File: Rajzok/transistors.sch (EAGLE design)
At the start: 17 parts, among them Q1 TP0602N2, Q2 TP0602N2, Q3 SUP75N06-08, Q4 SUP75N06-08

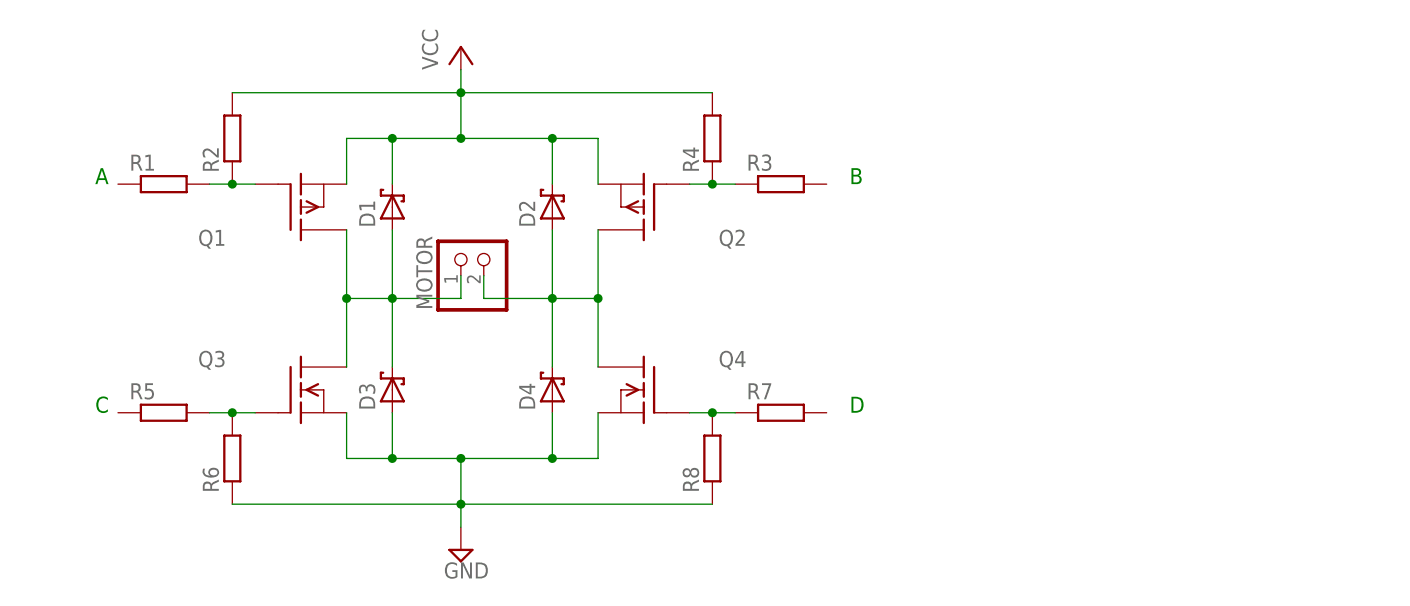
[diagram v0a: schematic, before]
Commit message: Rajzok 2017
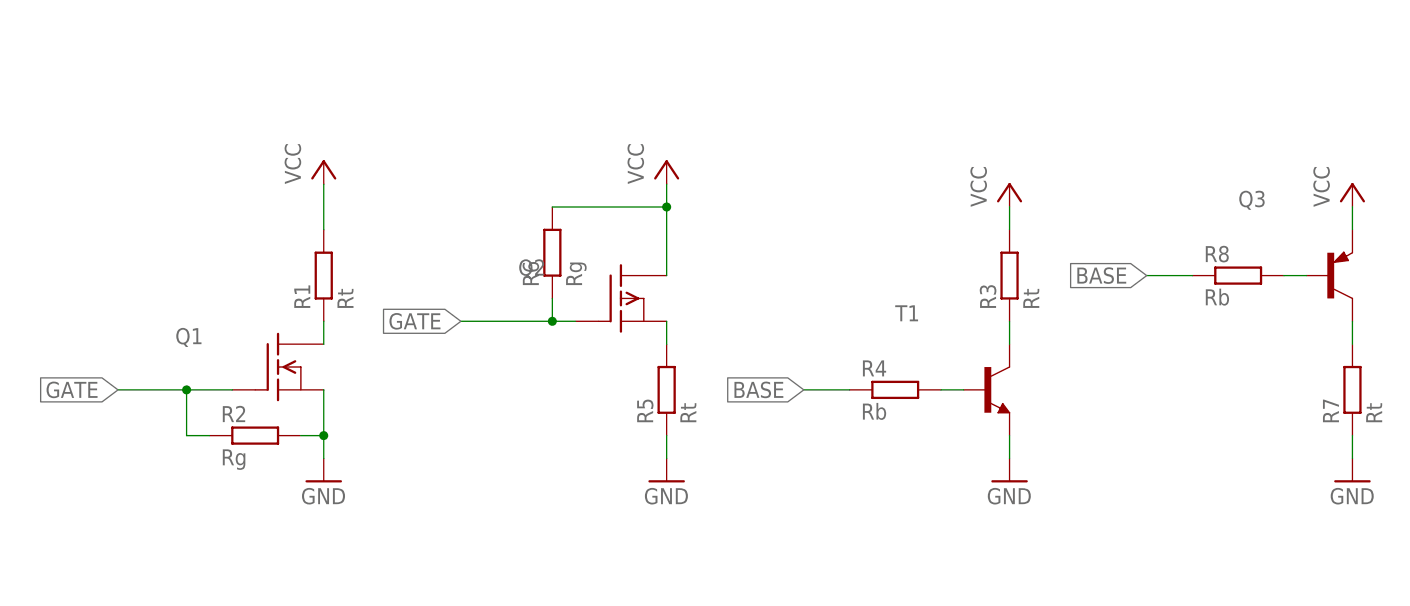
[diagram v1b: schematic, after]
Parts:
- removed D1, D2, D3, D4: 1N6267A, diode:1N6267A
- removed MOTOR: (no value), pinhead:PINHD-1X2
- removed Q4: SUP75N06-08, transistor-fet:SUP75N06-08
- added T1: 2N2219, transistor:2N2219
- Q1: value TP0602N2 -> BSS97; device transistor-fet:TP0602N2 -> transistor-fet:BSS97
- Q2: value TP0602N2 -> BSS92; device transistor-fet:TP0602N2 -> transistor-fet:BSS92
- Q3: value SUP75N06-08 -> 2N3576; device transistor-fet:SUP75N06-08 -> transistor-pnp:2N3576
- R1, R3, R5, R7: value (none) -> Rt; device rcl:R-EU_0204/7 -> rcl:R-EU_0207/15
- R2, R6: value (none) -> Rg; device rcl:R-EU_0204/7 -> rcl:R-EU_0207/15
- R4, R8: value (none) -> Rb; device rcl:R-EU_0204/7 -> rcl:R-EU_0207/15
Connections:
- removed net N$2: D2.A, D4.C, MOTOR.2, Q2.D, Q4.D
- removed net N$5: Q4.G, R7.1, R8.2
- new net BASE: R4.1, R8.1
- new net GATE: Q1.G, Q2.G, R2.1, R6.1
- new net N$10: Q3.B, R8.2
- new net N$6: Q2.S, R5.2
- net GND: now also Q1.S, R2.2, R5.1, R7.1, T1.E; no longer D3.A, D4.A, Q3.S, Q4.S, R6.1, R8.1
- net N$1: now also Q1.D, R1.1; no longer Q1.G, R1.2, R2.1
- net N$3: now also T1.C; no longer Q2.G, R4.1
- net N$4: now also R4.2, T1.B; no longer Q3.G, R5.2, R6.2
- net N$9: now also Q3.C, R7.2; no longer D1.A, D3.C, MOTOR.1, Q1.D, Q3.D
- net VCC: now also Q2.D, Q3.E, R1.2, R3.2, R6.2; no longer D1.C, D2.C, Q1.S, Q2.S, R2.2, R4.2
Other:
- note removed: "A"
- note removed: "B"
- note removed: "C"
- note removed: "D"
- moved on the sheet: Q1, Q2, R1, R2, R3, R4, R5, R6, R7, R8
